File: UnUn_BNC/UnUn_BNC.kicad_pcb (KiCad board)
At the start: 2 copper layers, 37.3 x 61.1 mm, 18 parts, among them J3 B_THT_Pad, J4 B_SMD_PAD, J5 A_THT_Pad, J6 A_SMD_PAD, U2 Core

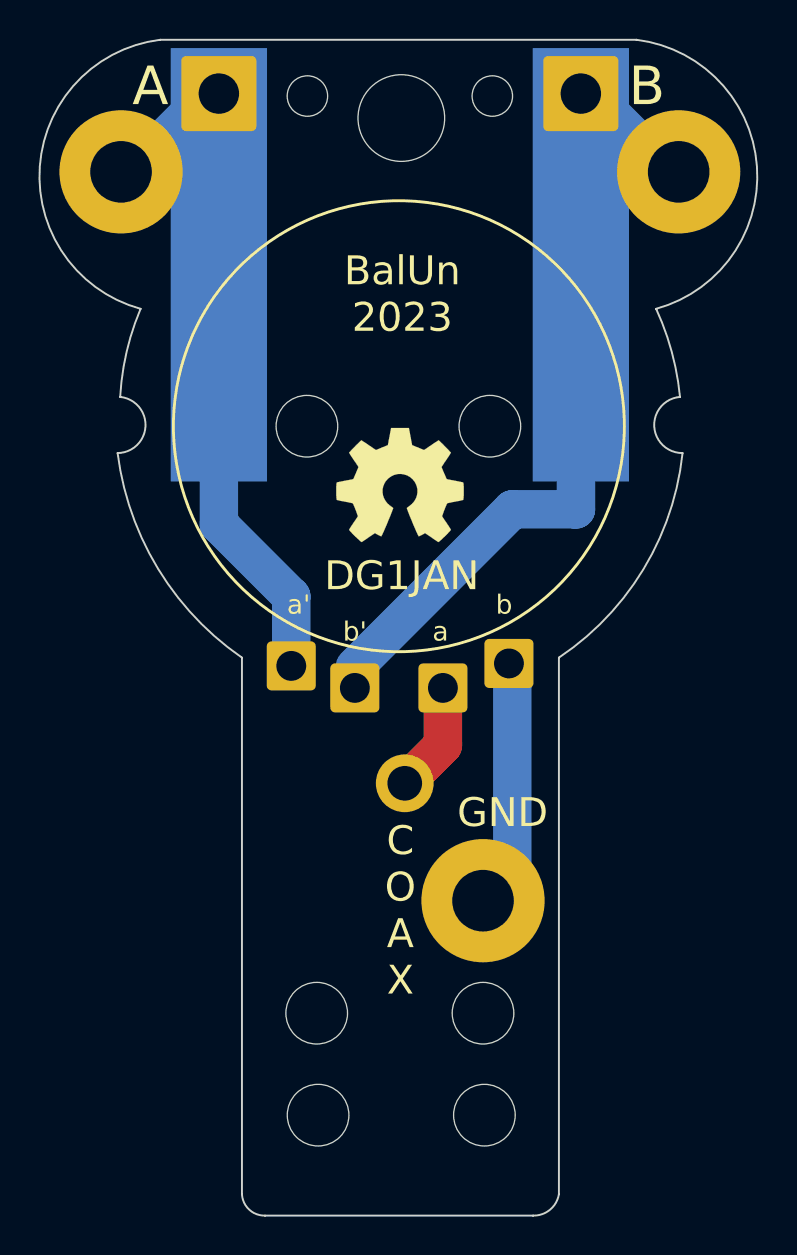
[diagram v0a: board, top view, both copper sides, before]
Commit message: Add files via upload
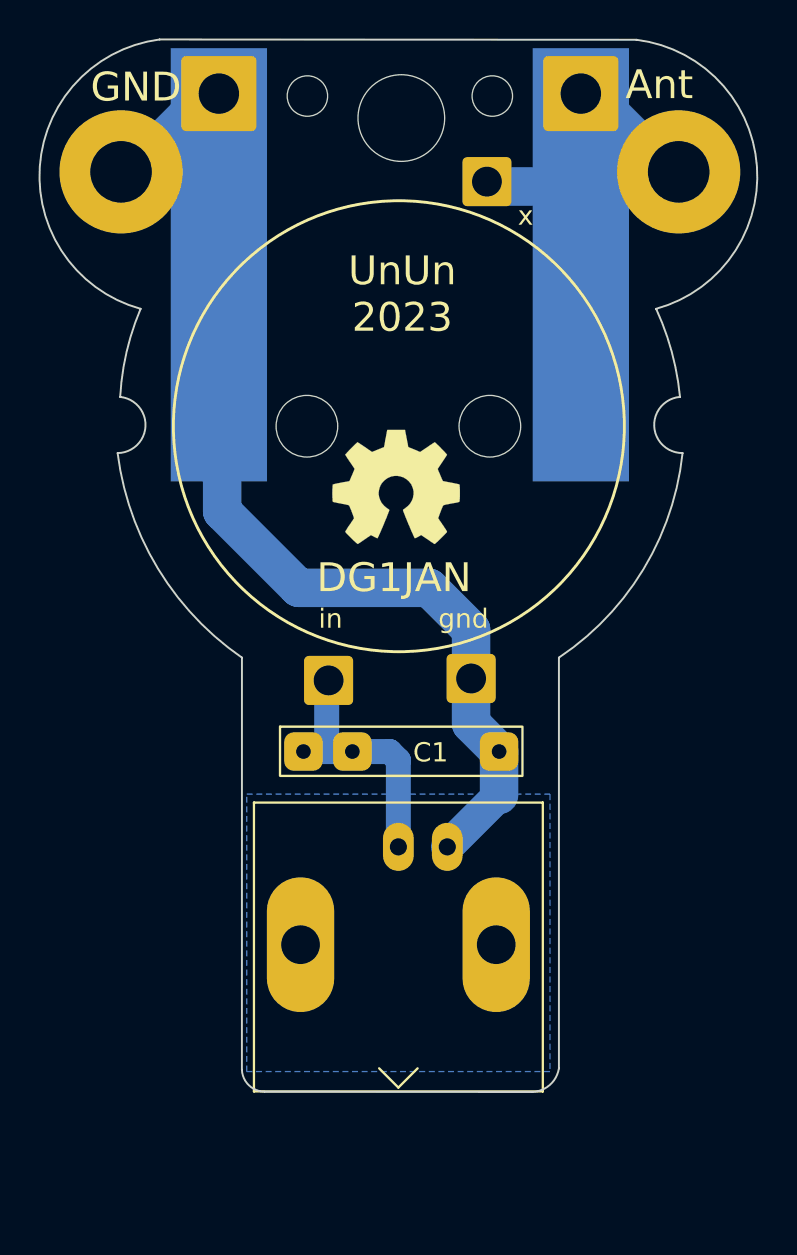
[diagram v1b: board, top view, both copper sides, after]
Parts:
- removed ? (x2): , 
- removed the REF** at (122.0, 101.3)
- removed the REF** at (113.3, 96.0)
- removed the REF** at (113.4, 101.3)
- removed the REF** at (121.9, 96.0)
- added C1: 100pF, UniBalunLibrary:THT_cap, F.Cu at (117.7, 82.4)
- added J1: BNC, Connector_Coaxial:BNC_Amphenol_B6252HB-NPP3G-50_Horizontal, F.Cu at (117.5, 87.4)
- moved REF** 0.22 mm to (117.4, 68.7)
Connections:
- H1 pad 1: (no net) -> Net-(H1-Pad1)
- H2 pad 1: (no net) -> GND
- J3 pad 1: (no net) -> Net-(H1-Pad1)
- J4 pad 1: (no net) -> Net-(H1-Pad1)
- J5 pad 1: (no net) -> GND
- J6 pad 1: (no net) -> GND
- U2 pad 1: (no net) -> GND
- U2 pad 4: (no net) -> Net-(C1-Pad1)
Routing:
- net (no net): track 111.0 -> 0.00 mm
- net GND: track 0.00 -> 65.2 mm
- net Net-(H1-Pad1): track 0.00 -> 32.5 mm
- net Net-(C1-Pad1): track 0.00 -> 13.4 mm
- added copper zone on B.Cu, net GND
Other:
- board size 37.3 x 61.1 mm -> 37.3 x 54.6 mm
- board text added: "Ant"
- board text added: "UnUn 2023"
- board text removed: "A"
- board text removed: "B"
- board text removed: "BalUn 2023"
- board text removed: "C O A X"
